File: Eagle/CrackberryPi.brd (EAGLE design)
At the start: 85 x 86 mm, 75 parts, among them IC1 REG1117, IC2 24C02CSM, Q2 FDN360P, X1 53261-02, X2 057-040-1, X5 FH12-50S-0.5SH

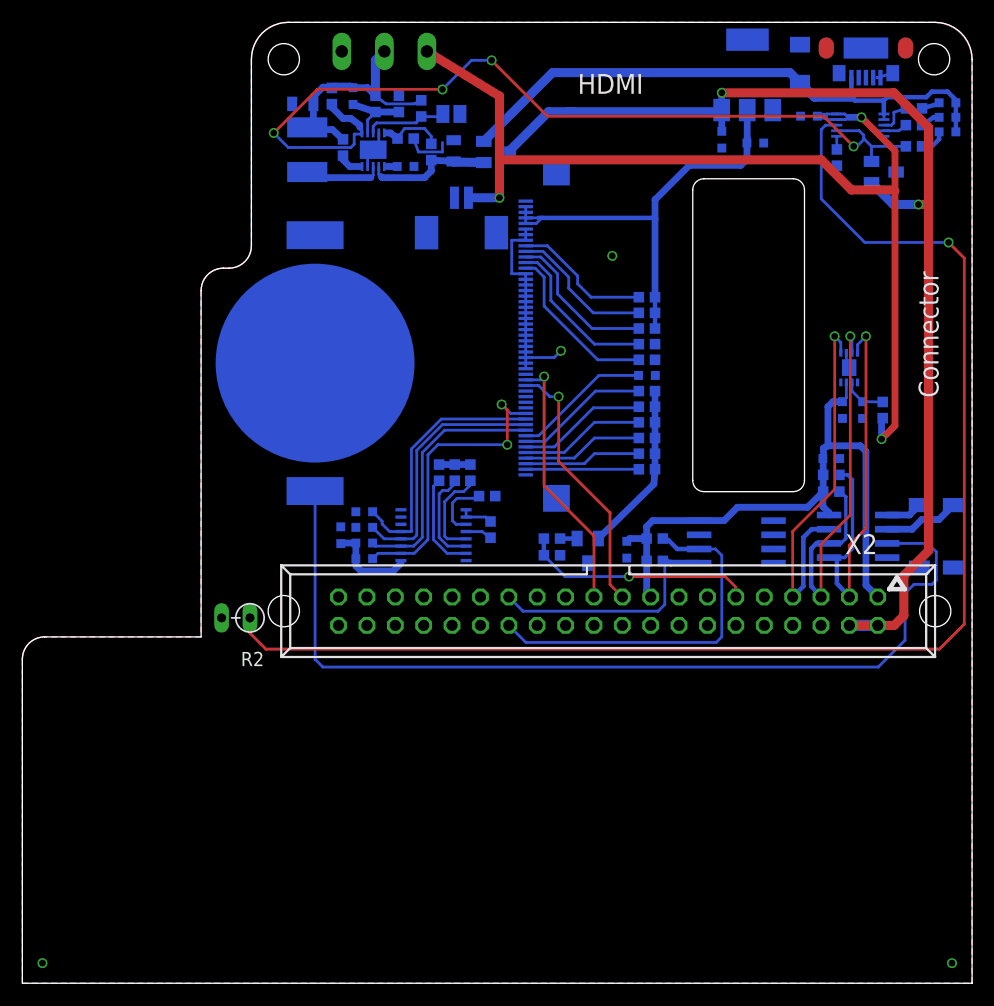
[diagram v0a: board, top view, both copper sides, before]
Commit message: finalizing pcb first proto
schematics, library parts and gerber rar
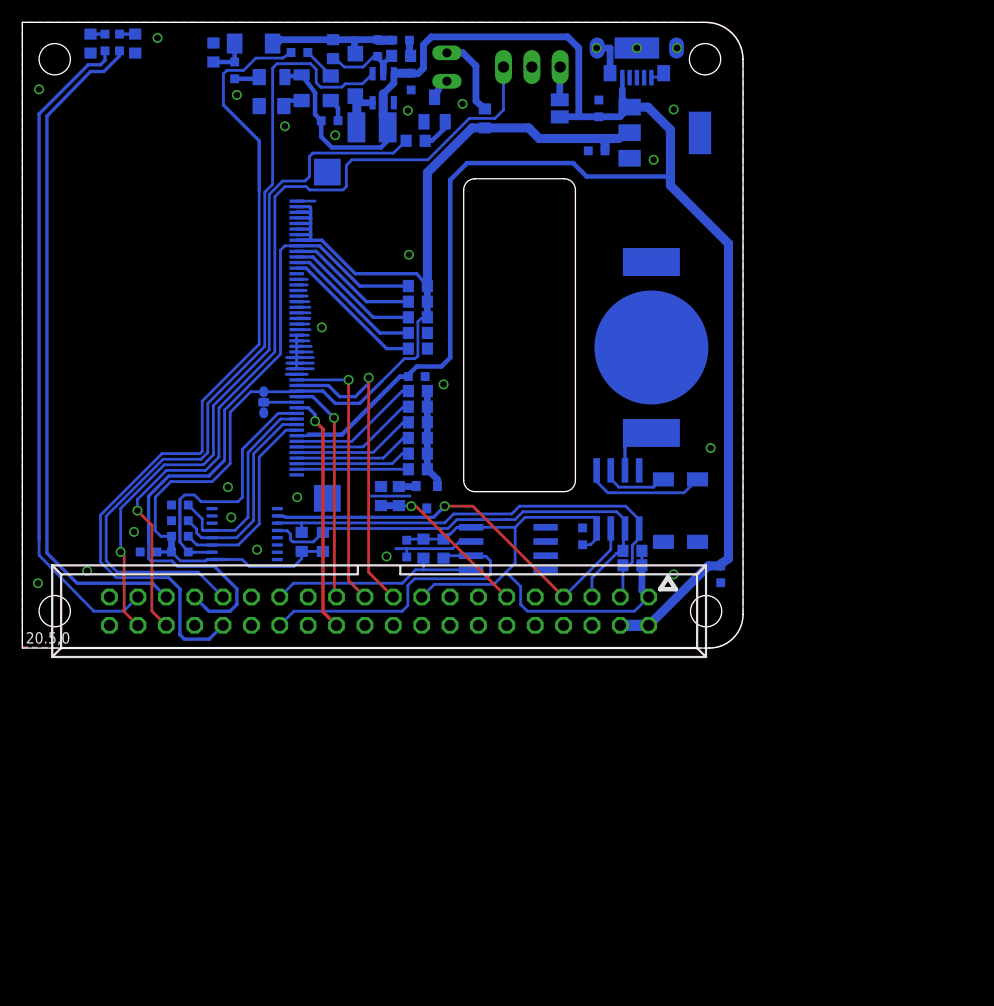
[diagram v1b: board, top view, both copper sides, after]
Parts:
- removed C10: 1mf, rcl:C0603
- removed C11: 10nf, rcl:C0603
- removed C12, C15: 0.1mf, rcl:C0603
- removed C16: 22mf, rcl:C0805
- removed C17: 10mf, rcl:C0805
- removed D2: (no value), diode:SOD80C
- removed D3: BAS40-05, diode:SOT23
- removed L2: (no value), rcl:L4532P
- removed LED1, LED2, LED3: (no value), eagle-ltspice:LED_SML0603
- removed Q2: FDN360P, transistor-power:SUPER-SOT3
- removed R10, R27: 1k, rcl:R0603
- removed R11, R8, R9: 470, rcl:R0603
- removed R12, R26, R28, R29, R34, R35, R7: 10k, rcl:R0603
- removed R30, R32: 2m, rcl:R0603
- removed R31, R33: 220k, rcl:R0603
- removed S1: (no value), switch:255SB
- removed SJ1: (no value), jumper:SJ
- removed U$1: TSC2046, tsc2046:TSSOP16
- removed U$7: MAX17043, MAX17043:DFN-2X3
- removed U$8: TPS61200, TPS61200:MCP73833
- removed X1: 53261-02, con-molex:53261-02
- added C19: 4.7mf, rcl:C0603
- added C20: 68pf, rcl:C0603
- added C21, C23: 470pf, rcl:C0603
- added C22: 0.1mf, rcl:C0603
- added C6: 10mf, rcl:C0603
- added D1: (no value), diode:SOD123
- added D4: 1N759, diode:SOD80C
- added D5: SFH482, led:SFH482
- added JMP1: 0R-JUMPC, jump-0r-smd:C0R-JMP
- added L1: 8.2mH, rcl:R1210
- added LED4, LED5: (no value), eagle-ltspice:LED_SML0603
- added R36: 1.3m, rcl:R0603
- added R37: 110k, rcl:R0603
- added R38, R39: 30, rcl:R0603
- added R40: 1k, rcl:R0603
- added R41, R42: 10k, rcl:R0603
- added SJ2: (no value), jumper:SJ
- added T1: BC847, transistor:SOT23
- added U$10, U$3: MAX2650, max2650:SOT143-W
- added U$2: NCP1406, ncp1406:SOT23-5L
- added X3: C-GRID-03-70543, con-molex:70543-03
- C13, C14: value 0.1mf -> 4.7mF
- C8: value (none) -> 0.1mf
- C9: value (none) -> 1mf
- Q1: value (none) -> IRLML5203; device semicon-smd-ipc:SOT23 -> transistor-power:MICRO3
- R2: value THERMISTOR-2,5 -> 10k; device varistor:RS-2,5 -> rcl:R0603
- U$4: value MCP73833 -> CR1216; device mcp73833:MSOP10 -> cr1216:CR1216
- U$6: value CR2032 -> TSC2007; device cr2032:CR2032 -> tsc2046:TSSOP16
- moved Q1 50.2 mm to (36.2, 13.5), turned to 180 degrees
- moved C8 41.8 mm to (62.5, 6.60), turned to 270 degrees
- moved U$4 27.3 mm to (56.3, 26.9), turned to 90 degrees
- moved C1 23.3 mm to (50.1, 10.0), turned to 90 degrees
- moved Q3 23.0 mm to (58.9, 12.3)
- moved U$5 21.8 mm to (53.3, 13.3), turned to 180 degrees
- moved R5 20.7 mm to (35.9, 8.90), turned to 90 degrees
- moved C9 20.6 mm to (35.3, 24.3)
- moved R13 20.5 mm to (35.4, 32.4)
- moved R14 20.5 mm to (35.4, 31.0)
- moved R15 20.5 mm to (35.4, 29.6)
- moved R16 20.5 mm to (35.4, 28.2)
- moved R17 20.5 mm to (35.4, 26.8)
- moved R18 20.5 mm to (35.4, 23.0)
- moved R19 20.5 mm to (35.4, 21.6)
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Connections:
- net GPIO21 renamed AVALANCHE_ENABLE
- removed net +5V/4: C9.1, X5.43
- removed net 2046_BUSY: R34.1, U$1.13
- removed net 2046_CS: R6.1, U$1.15
- removed net BAT+: C8.1, R27.1, S1.3, U$4.10, U$4.9, X1.1
- removed net CS: X5.38
- removed net ENABLE_STEPUP: Q1.2, R11.2, R28.1, U$4.7, U$8.6
- removed net GPIO12: X2.32
- removed net GPIO13: X2.33
- removed net GPIO16: X2.36
- removed net GPIO20: X2.38
- removed net GPIO6: X2.31
- removed net N$1: Q3.1, U$5.2
- removed net N$13: R8.2, U$4.3
- removed net N$14: LED1.C, R8.1
- removed net N$15: R9.2, U$4.4
- removed net N$17: LED3.C, R11.1
- removed net N$18: LED2.C, R9.1
- removed net N$19: R10.2, U$4.6
- removed net N$2: Q3.4, U$5.1
- removed net N$21: R2.1, U$4.8
- removed net N$22: R29.1, SJ1.2, U$8.8
- removed net N$23: C12.2, R30.1, R31.2, U$8.7
- removed net N$24: L2.2, U$8.3
- removed net N$26: C15.1, U$8.1
- removed net N$27: R32.1, R33.2, U$8.10
- removed net N$28: D2.C, D3.2, LED1.A, LED2.A, LED3.A, U$4.1, U$4.2, U$9.1_+5V
- removed net N$3: U$5.3, U$6.+
- removed net N$5: C10.1, R27.2, U$7.2
- removed net N$6: C16.1, D3.1, R32.2, U$8.2
- removed net PENIRQ: R7.1, U$1.11
- removed net RD: X5.35
- removed net RST: R13.1, X5.9
- removed net VBAT: C12.1, C17.1, L2.1, R26.2, R28.2, R29.2, R30.2, S1.2
- new net +15V: C19.1, C20.1, D1.C, D4.C, R36.2
- new net BASE: R40.1, T1.1
- new net COLLECTOR: D5.K, T1.3
- new net DISPLAY_RESET: R13.1, X2.33, X5.9
- new net EMITTER: T1.2
- new net FB: C20.2, R36.1, R37.2, U$2.2
- new net IN_1: C21.2, U$3.1
- new net IR_RX: X2.36, X3.1
- new net IR_TX: R40.2, X2.38
- new net LX: D1.A, L1.2, U$2.5
- new net N$16: C21.1, D4.A, R38.2
- new net N$30: D5.A, R39.1
- new net N$35: LED4.C, R41.2
- new net N$36: LED5.C, R42.2
- new net OUT1_IN2: U$10.1, U$3.3
- new net OUT2: C23.2, U$10.3
- new net RANDOM: C23.1, X2.32
- new net STEPUP_ENABLE: U$2.1, X2.31
- new net VBAT+: U$4.+, U$5.3
- new net X1_RTC: Q3.1, U$5.1
- new net X2_RTC: Q3.4, U$5.2
- net +3V3: now also C14.1, C2.1, C3.1, C7.1, IC1.2, JMP1.1, R13.2, R14.2, R15.2, R2.2, R39.2, R6.2, U$6.1, X5.2, X5.3, X5.35, X5.4, X5.5, X5.6, X5.7, X5.8; no longer C1.1, C11.1, C5.1, IC2.8, R1.2, R3.2, R4.2, R5.2, U$5.8, U$7.3, X2.1, X2.17
- net +5V: now also C22.2, C6.1, C8.1, C9.1, L1.1, SJ2.2, U$10.4, U$2.3, U$3.4, U$9.1_+5V, X5.43; no longer D3.3, Q1.1
- net CE0: now also X5.38
- net D/C: now also JMP1.2
- net GND: now also C19.2, C22.1, C6.2, JMP1.3, R37.1, R38.1, R41.1, R42.1, U$10.2, U$2.4, U$3.2, U$4.GND, U$6.13, U$6.14, U$6.16, U$6.6, X3.2; no longer C10.2, C11.2, C15.2, C16.2, C17.2, D2.A, Q2.3, R10.1, R2.2, R31.1, R33.1, R7.2, SJ1.1, U$1.6, U$1.7, U$1.8, U$4.5, U$6.GND, U$7.1, U$7.4, U$7.6, U$7.EXP, U$8.4, U$8.9, U$8.GND, U$9.4_ID, U$9.GND3, U$9.GND4, X1.2, X5.6, X5.7, X5.8
- net GPIO19: now also LED4.A
- net GPIO26: now also LED5.A
- net INT: now also U$6.10; no longer U$7.5
- net MISO: no longer R35.1, U$1.12
- net MOSI: no longer R12.1, U$1.14
- net N$12: now also Q1.2; no longer Q2.2
- net N$20: now also Q1.1; no longer Q2.1
- net N$4: now also SJ2.1, X3.3; no longer R26.1, U$8.5
- net SCK: no longer U$1.16
- net SCL_3V3: now also R6.1, U$6.12; no longer U$7.7
- net SDA_3V3: now also R2.1, U$6.11; no longer U$7.8
- net TOUCH_X+: now also U$6.2; no longer U$1.2
- net TOUCH_X-: now also U$6.4; no longer U$1.4
- net TOUCH_Y+: now also U$6.3; no longer U$1.3
- net TOUCH_Y-: now also U$6.5; no longer U$1.5
- net VCC: now also C1.1, C5.1, IC2.8, R1.2, R3.2, R4.2, R5.2, U$5.8, X2.1, X2.17; no longer C14.1, C2.1, C3.1, C7.1, IC1.2, R12.2, R13.2, R14.2, R15.2, R34.2, R35.2, R6.2, U$1.1, U$1.10, U$1.9, X5.2, X5.3, X5.4, X5.5
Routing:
- net N$21: track 122.3 -> 0.00 mm, vias 1 -> 0
- net BAT+: track 100.7 -> 0.00 mm, vias 3 -> 0
- net N$3: track 83.8 -> 0.00 mm
- net ENABLE_STEPUP: track 81.2 -> 0.00 mm, vias 4 -> 0
- net RANDOM: track 0.00 -> 76.4 mm
- net IR_RX: track 0.00 -> 75.5 mm, vias 0 -> 1
- net STEPUP_ENABLE: track 0.00 -> 75.2 mm
- net +5V: track 102.1 -> 168.9 mm, vias 2 -> 0
- net +3V3: track 56.5 -> 119.5 mm
- net DISPLAY_RESET: track 0.00 -> 62.7 mm
- net IR_TX: track 0.00 -> 62.0 mm, vias 0 -> 1
- net GPIO19: track 0.00 -> 60.6 mm
- net GPIO26: track 0.00 -> 59.7 mm
- net N$28: track 52.8 -> 0.00 mm
- net VBAT: track 24.2 -> 0.00 mm
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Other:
- board size 85 x 86 mm -> 64.5 x 56 mm
- board text added: "20.5,0"
- board text added: "CrackberryPi v1.0.1"
- board text removed: "Connector"
- board text removed: "HDMI"
